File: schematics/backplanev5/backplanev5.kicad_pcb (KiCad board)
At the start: 2 copper layers, 150 x 103.8 mm, 28 parts, among them J12 Conn_01x02, J13 Conn_01x02, J14 Conn_01x02

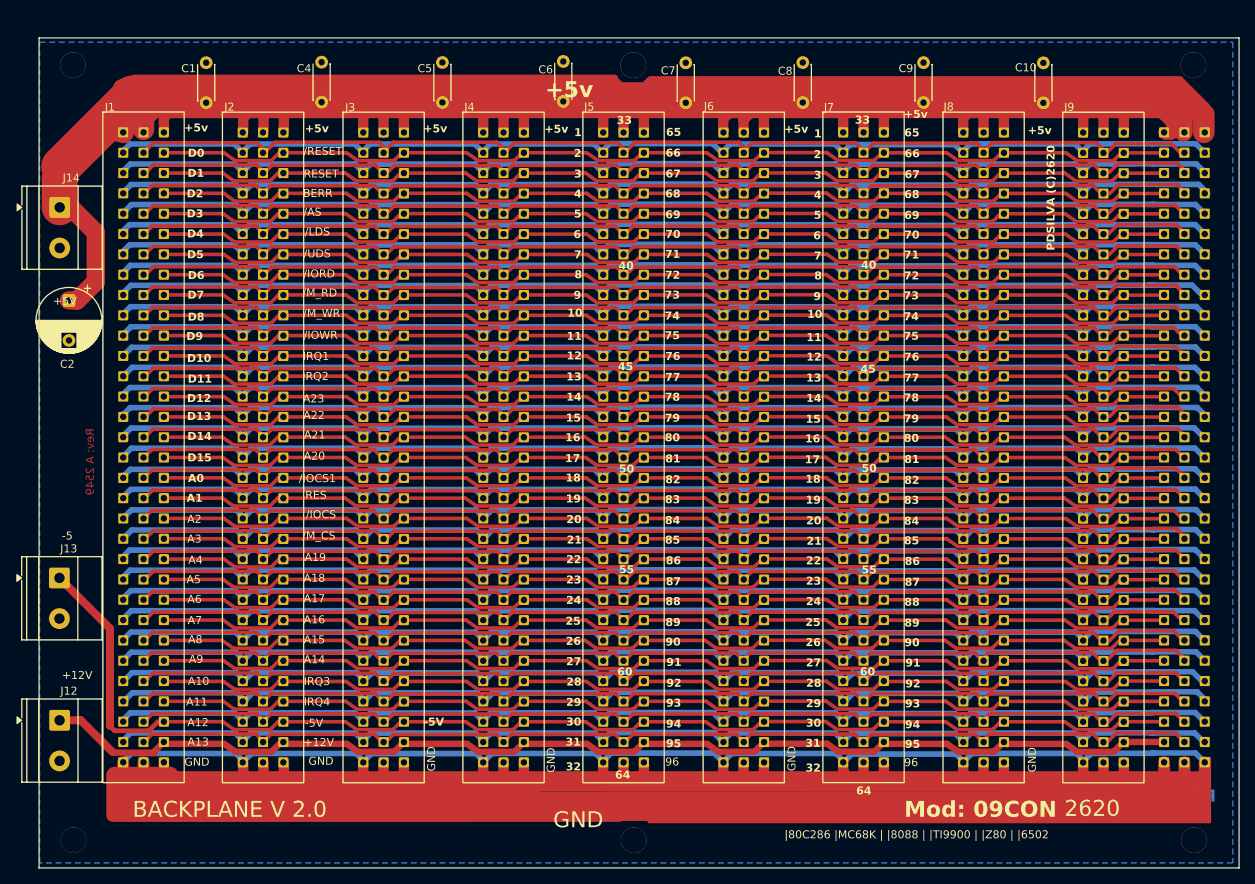
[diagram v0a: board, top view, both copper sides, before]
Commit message: Terminado o DRC
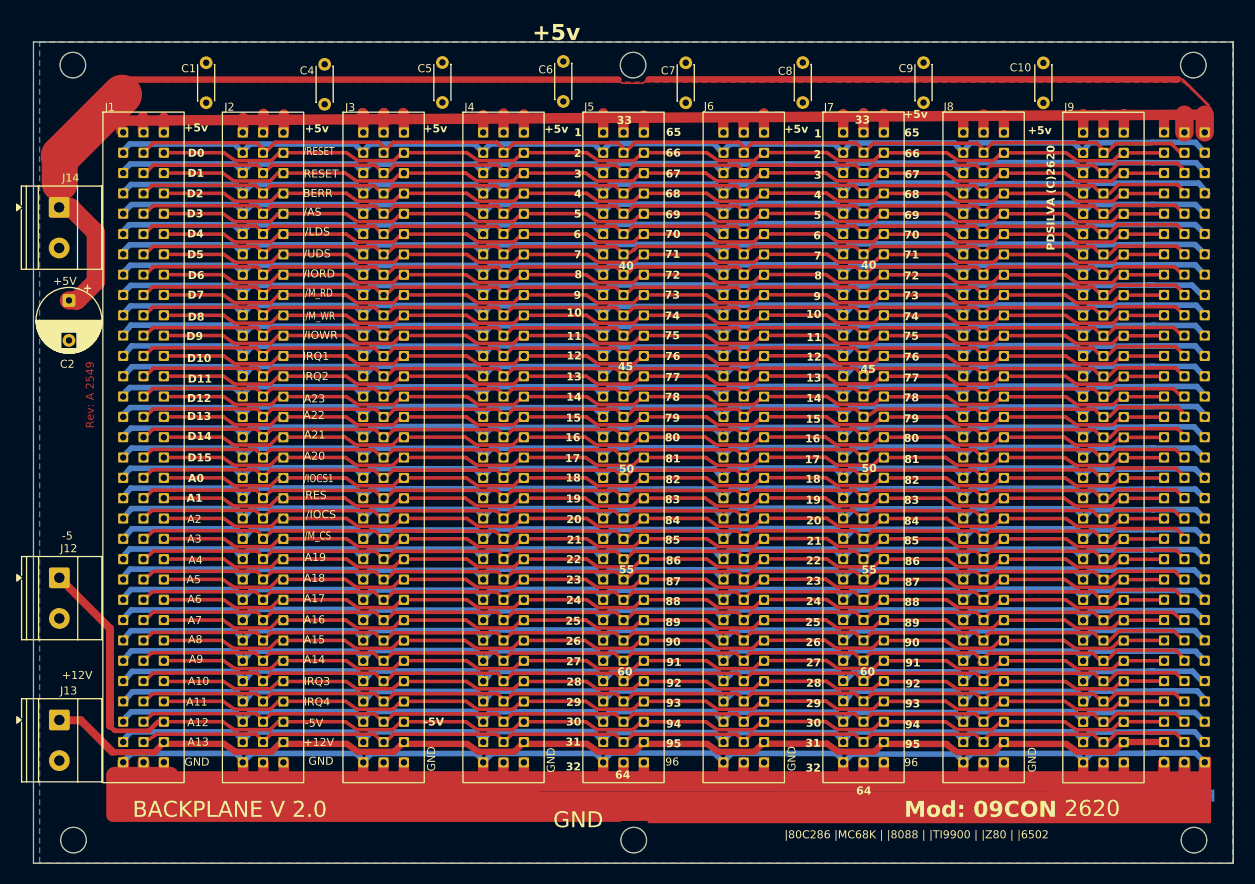
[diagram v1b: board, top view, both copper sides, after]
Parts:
- moved J12 17.8 mm to (18.3, 85.7)
- moved J13 17.8 mm to (18.3, 103.4)
- moved C4 0.47 mm to (51.5, 26.5)
- moved J14 0.07 mm to (18.3, 39.4)
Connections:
- C4 pad 1: unconnected-(C4-Pad1) -> /backplane/+5V
- C4 pad 2: unconnected-(C4-Pad2) -> GND
- C5 pad 1: unconnected-(C5-Pad1) -> /backplane/+5V
- C5 pad 2: unconnected-(C5-Pad2) -> GND
- J12 pad 1: /backplane/+12V -> /backplane/-5V
- J13 pad 1: /backplane/-5V -> /backplane/+12V
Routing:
- net /backplane/+5V: track 506.5 -> 236.4 mm
- net /backplane/A8: track 142.4 -> 145.1 mm
- net /backplane/A10: track 143.0 -> 145.6 mm
- net /backplane/A9: track 142.7 -> 145.1 mm
- net /backplane/A11: track 142.7 -> 145.0 mm
- net /backplane/D8: track 142.7 -> 144.4 mm
- net /backplane/A12: track 142.7 -> 144.4 mm
- net /backplane/D10: track 142.7 -> 144.3 mm
- net /backplane/D11: track 142.7 -> 144.0 mm
- net /backplane/A0: track 142.7 -> 144.0 mm
- net /backplane/A2: track 142.7 -> 144.0 mm
- net /backplane/D9: track 142.7 -> 144.0 mm
- net /backplane/A13: track 142.7 -> 143.9 mm
- net /backplane/D12: track 142.7 -> 143.9 mm
- net /backplane/A3: track 142.7 -> 143.8 mm
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- added copper zone on F.Cu, net /backplane/+5V
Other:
- board size 150 x 103.8 mm -> 150 x 102.7 mm
